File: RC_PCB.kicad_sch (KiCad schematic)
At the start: 19 parts, among them SW1 SW_Push, SW2 SW_Push, SW3 SW_Push, SW4 SW_Push, U1 RFM9x, U2 Teensy4.0, U3 128x64_OLED, U4 Joystick, U5 Joystick

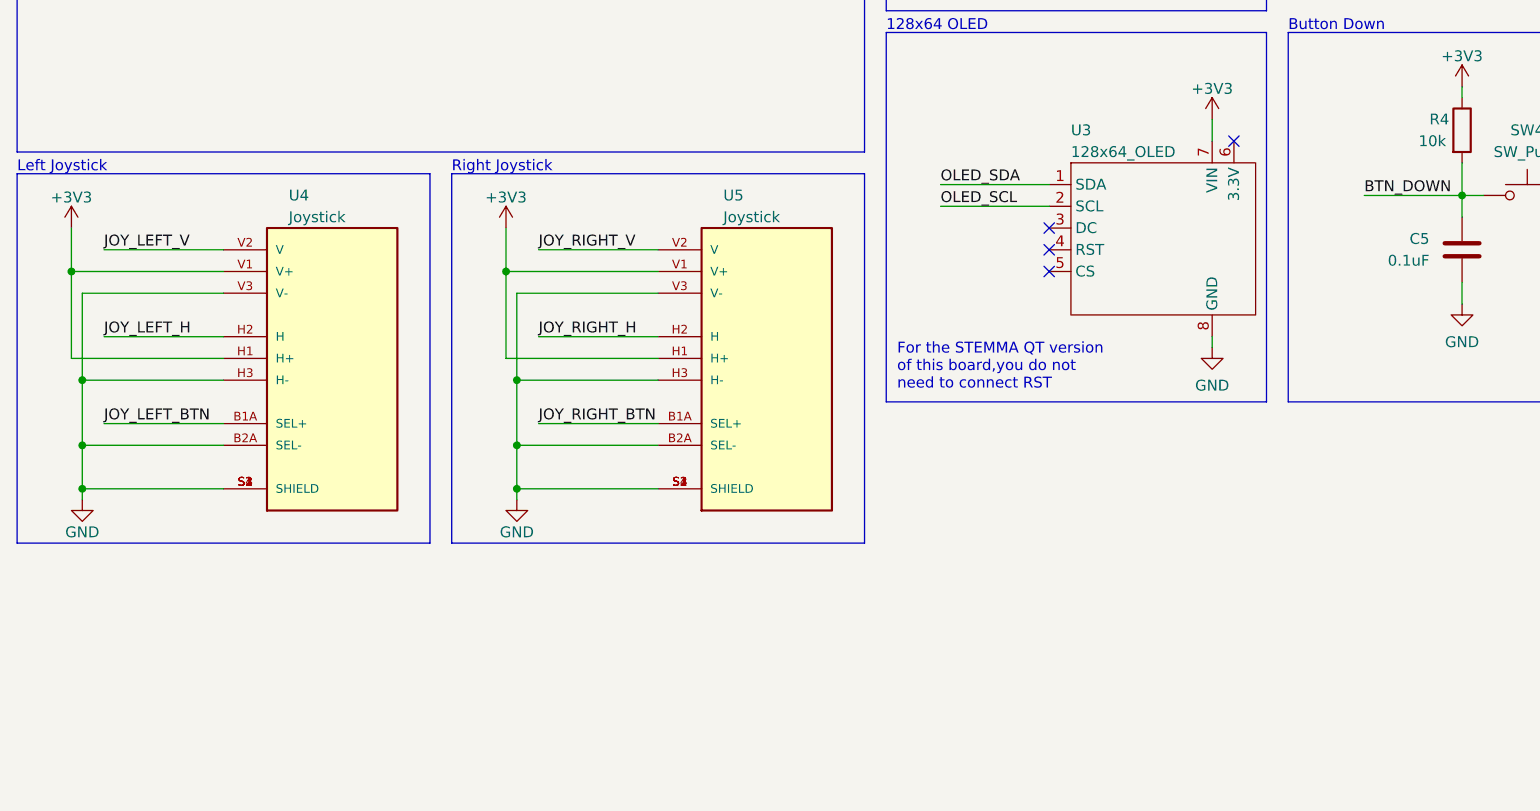
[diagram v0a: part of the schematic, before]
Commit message: initial layout complete
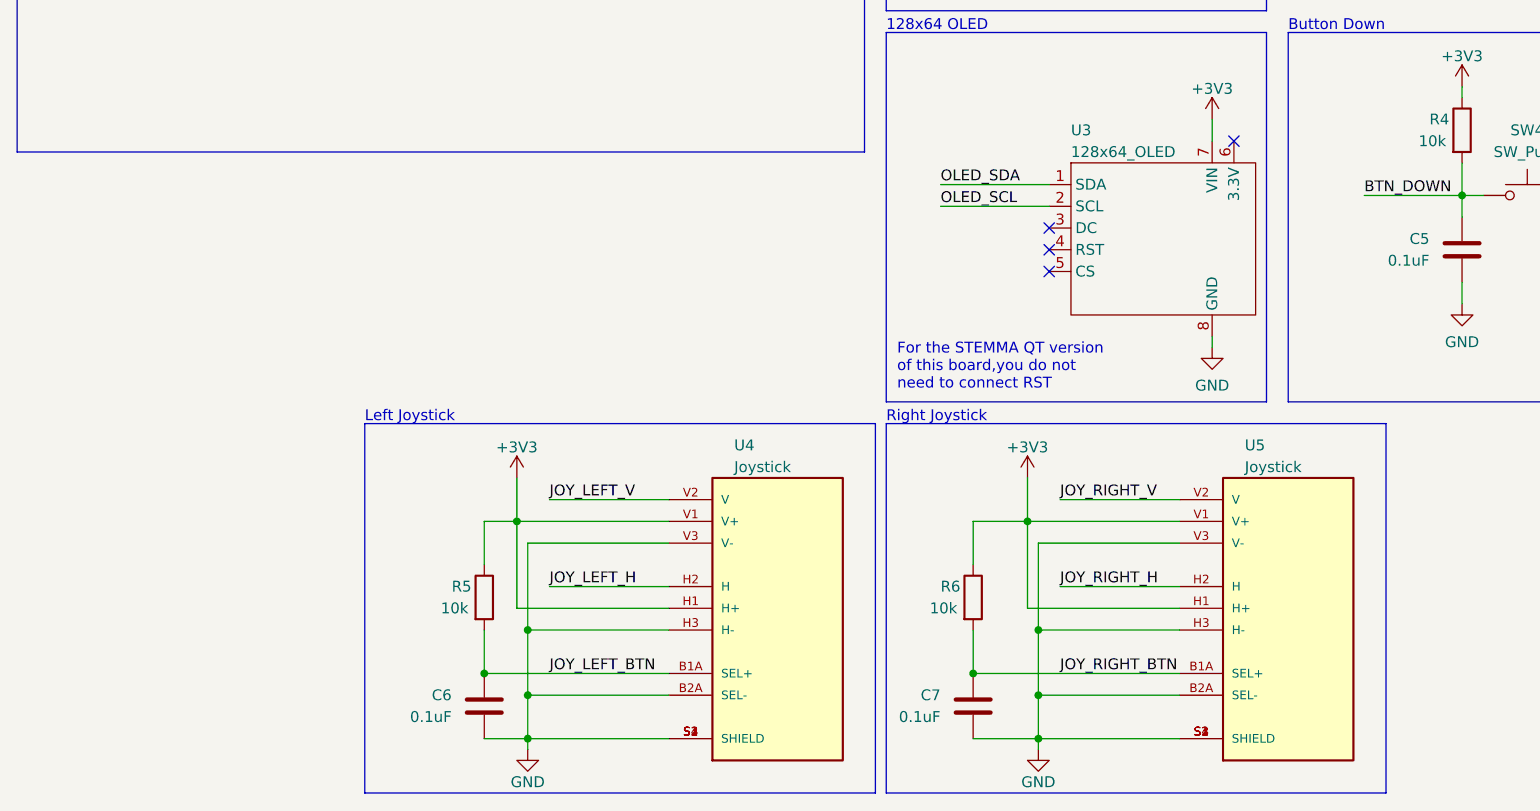
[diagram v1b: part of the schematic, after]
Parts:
- added C6, C7: 0.1uF, Capacitor_SMD:C_0805_2012Metric_Pad1.18x1.45mm_HandSolder, symbol Device:C
- added R5, R6: 10k, Resistor_SMD:R_0805_2012Metric_Pad1.20x1.40mm_HandSolder, symbol Device:R
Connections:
- net +3V3: now also R5.1, R6.1
- net GND: now also C6.2, C7.2
- net JOY_LEFT_BTN: now also C6.1, R5.2
- net JOY_RIGHT_BTN: now also C7.1, R6.2
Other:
- moved on the sheet: U4, U5
